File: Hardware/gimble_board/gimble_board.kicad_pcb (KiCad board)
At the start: 2 copper layers, 124.5 x 95.9 mm, 97 parts, among them J1 Test_Point, J2 Test_Point, J3 Test_Point, J4 Test_Point, Q1 Q_NMOS_GDS, Q2 Q_NMOS_GDS, Q3 Q_NMOS_GDS, Q4 Q_NMOS_GDS, Q5 Q_NMOS_GDS, Q6 Q_NMOS_GDS, Q7 Q_NMOS_GDS, Q8 Q_NMOS_GDS, SW1 SW_Push, SW2 SW_Push, SW3 SW_Push, SW4 SW_Push, SW5 SW_Push, SW6 SW_Push, SW7 SW_Push, SW8 SW_Push, SW9 SW_SPDT, U1 LM2576SX-3.3, U2 LM2576SX-5.0, U3 TM4C129E_Launchpad

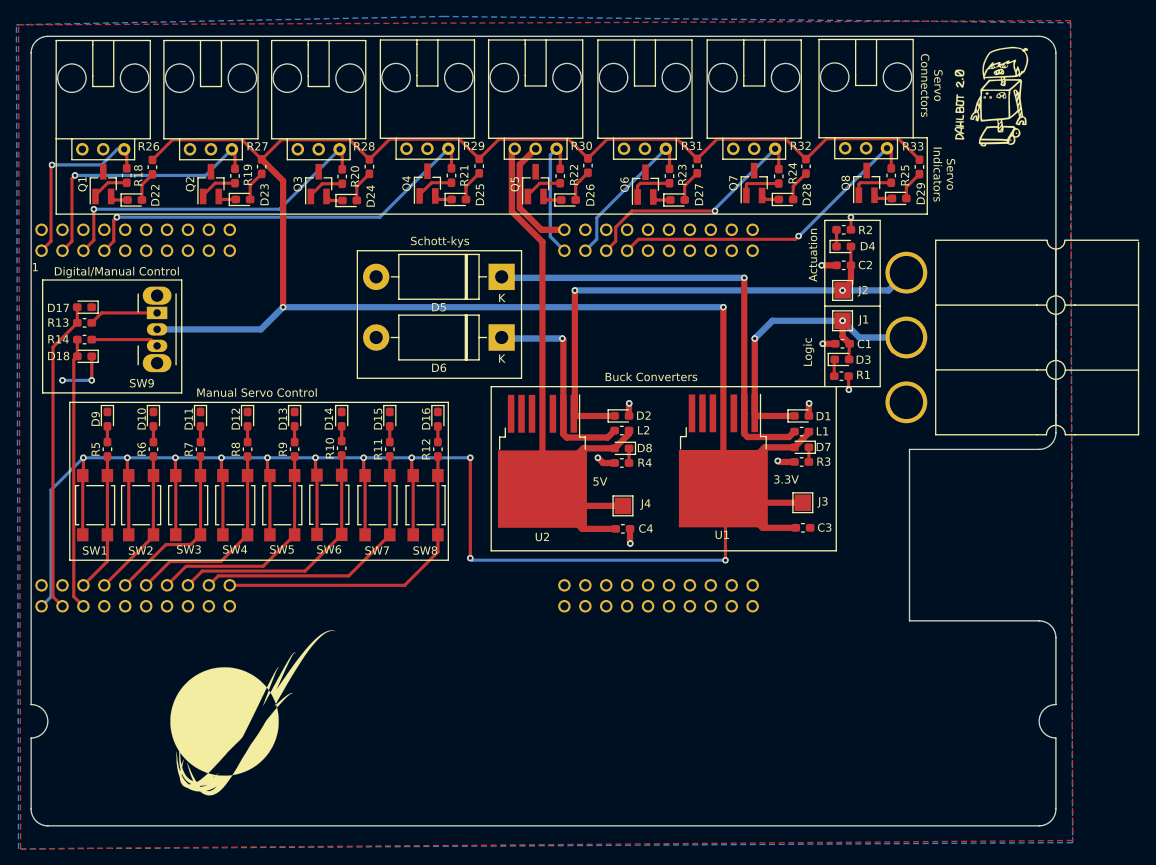
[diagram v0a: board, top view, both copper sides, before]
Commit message: layout 9
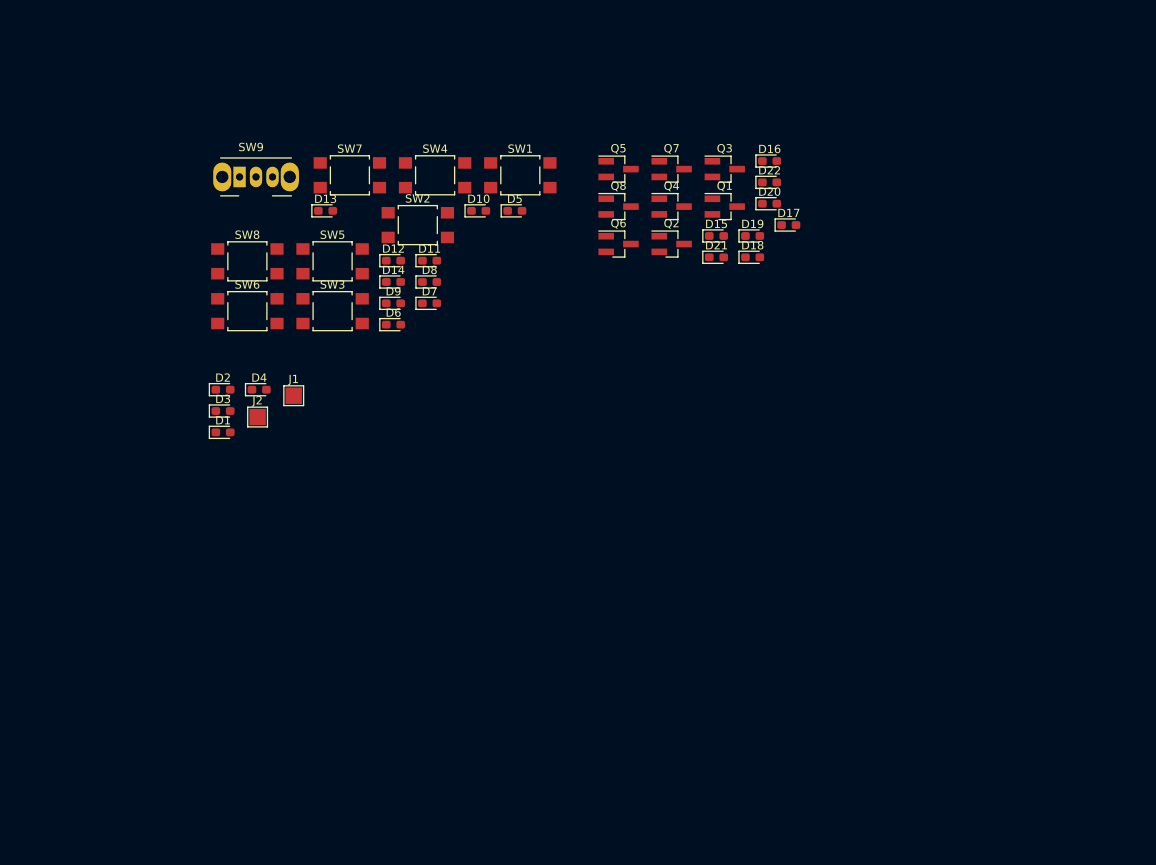
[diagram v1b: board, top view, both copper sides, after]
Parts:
- removed C1, C2: 100uF, Capacitor_SMD:C_0603_1608Metric_Pad1.05x0.95mm_HandSolder
- removed C3, C4: 1000uF, Capacitor_SMD:C_0603_1608Metric_Pad1.05x0.95mm_HandSolder
- removed Conn1: AndersonPP, MRDT_Connectors:Anderson_3_Horizontal_Side_by_Side
- removed Conn2, Conn3, Conn4, Conn5, Conn6, Conn7, Conn8, Conn9: Molex_SL_03, MRDT_Connectors:MOLEX_SL_03_Horizontal
- removed D23, D24, D25, D26, D27, D28, D29: LED, LED_SMD:LED_0603_1608Metric_Pad1.05x0.95mm_HandSolder
- removed G***: LOGO, MRDT_Silkscreens:0_MRDT_Logo_20mm
- removed G***: LOGO, MRDT_Silkscreens:2_Dahlbot_2.0
- removed J3, J4: Test_Point, TestPoint:TestPoint_Pad_2.0x2.0mm
- removed L1, L2: 100uH, Inductor_SMD:L_0603_1608Metric_Pad1.05x0.95mm_HandSolder
- removed R1, R2: 1k, Resistor_SMD:R_0603_1608Metric_Pad1.05x0.95mm_HandSolder
- removed R10, R11, R12, R13, R14, R26, R27, R28, R29, R3, R30, R31, R32, R33, R5, R6, R7, R8, R9: 330, Resistor_SMD:R_0603_1608Metric_Pad1.05x0.95mm_HandSolder
- removed R18, R19, R20, R21, R22, R23, R24, R25, R4: 500, Resistor_SMD:R_0603_1608Metric_Pad1.05x0.95mm_HandSolder
- removed U1: LM2576SX-3.3, Package_TO_SOT_SMD:TO-263-6
- removed U2: LM2576SX-5.0, Package_TO_SOT_SMD:TO-263-6
- removed U3: TM4C129E_Launchpad, MRDT_Shields:TM4C129E_Launchpad_FULL_THT_BOTTOM
- added D19: LED, LED_SMD:LED_0603_1608Metric_Pad1.05x0.95mm_HandSolder, F.Cu at (151.1, 52.8)
- added D20: LED, LED_SMD:LED_0603_1608Metric_Pad1.05x0.95mm_HandSolder, F.Cu at (153.2, 48.9)
- added D21: LED, LED_SMD:LED_0603_1608Metric_Pad1.05x0.95mm_HandSolder, F.Cu at (146.7, 55.4)
- D5, D6: value D_Schottky -> LED; footprint Diode_THT:D_DO-201AD_P15.24mm_Horizontal -> LED_SMD:LED_0603_1608Metric_Pad1.05x0.95mm_HandSolder
- moved D17 86.1 mm to (155.5, 51.5), turned to 0 degrees
- moved D18 82.0 mm to (151.1, 55.4), turned to 0 degrees
- moved D22 77.1 mm to (153.2, 46.3)
- moved Q1 75.5 mm to (147.7, 49.3), turned to 0 degrees
- moved D3 75.4 mm to (86.8, 74.1)
- moved D4 73.1 mm to (91.2, 71.5)
- moved J2 72.7 mm to (91.0, 74.8)
- moved D1 70.3 mm to (86.8, 76.7)
- moved J1 67.3 mm to (95.4, 72.2)
- moved SW1 65.4 mm to (122.9, 45.5), turned to 0 degrees
- moved Q2 56.4 mm to (141.3, 53.8), turned to 0 degrees
- moved D16 51.0 mm to (153.2, 43.7), turned to 0 degrees
- moved Q3 49.4 mm to (147.7, 44.7), turned to 0 degrees
- moved D2 48.5 mm to (86.8, 71.5)
- moved D7 48.5 mm to (111.9, 61.0), turned to 0 degrees
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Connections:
- D13 pad 2: Net-(D13-Pad2) -> Servo_Digital_Control
- D14 pad 2: Net-(D14-Pad2) -> Servo_Manual_Control
- D15 pad 1: GND -> Net-(D15-Pad1)
- D16 pad 1: GND -> Net-(D16-Pad1)
- D17 pad 1: GND -> Net-(D17-Pad1)
- D17 pad 2: Servo_Digital_Control -> Net-(D17-Pad2)
- D18 pad 1: GND -> Net-(D18-Pad1)
- D18 pad 2: Servo_Manual_Control -> Net-(D18-Pad2)
- D5 pad 1: Net-(D5-Pad1) -> GND
- D5 pad 2: GND -> Net-(D5-Pad2)
- D6 pad 1: Net-(D6-Pad1) -> GND
- D6 pad 2: GND -> Net-(D6-Pad2)
- D7 pad 1: Net-(D7-Pad1) -> GND
- D7 pad 2: +3V3 -> Net-(D7-Pad2)
- D8 pad 1: Net-(D8-Pad1) -> GND
- D8 pad 2: +5V -> Net-(D8-Pad2)
- Q1 pad 2: Net-(D22-Pad1) -> Net-(D15-Pad1)
- Q2 pad 2: Net-(D23-Pad1) -> Net-(D16-Pad1)
- Q3 pad 2: Net-(D24-Pad1) -> Net-(D17-Pad1)
- Q4 pad 2: Net-(D25-Pad1) -> Net-(D18-Pad1)
- Q8 pad 2: Net-(D29-Pad1) -> Net-(D22-Pad1)
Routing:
- net +3V3: track 449.7 -> 0.00 mm, vias 13 -> 0
- net +5V: track 86.1 -> 0.00 mm
- net Power_Input_Act: track 67.0 -> 0.00 mm, vias 2 -> 0
- net Net-(D5-Pad1): track 55.0 -> 0.00 mm, vias 1 -> 0
- net Servo_4_PWM: track 50.9 -> 0.00 mm, vias 1 -> 0
- net Power_Input_Log: track 43.5 -> 0.00 mm, vias 2 -> 0
- net Servo_3_PWM: track 41.0 -> 0.00 mm, vias 1 -> 0
- net Servo_8_AW: track 39.4 -> 0.00 mm, vias 1 -> 0
- net Servo_8_SW: track 38.6 -> 0.00 mm
- net Servo_Digital_Control: track 38.0 -> 0.00 mm
- net GND: track 37.1 -> 0.00 mm, vias 11 -> 0
- net Servo_7_SW: track 34.0 -> 0.00 mm
- net Servo_Manual_Control: track 33.0 -> 0.00 mm
- net Servo_2_PWM: track 32.7 -> 0.00 mm, vias 1 -> 0
- net Servo_6_SW: track 30.8 -> 0.00 mm
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- removed copper zone on B.Cu, net +5V
- removed copper zone on F.Cu, net GND
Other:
- board outline removed
- board text removed: "3.3V"
- board text removed: "5V"
- board text removed: "Actuation"
- board text removed: "Buck Converters"
- board text removed: "Digital/Manual Control"
- board text removed: "Logic"
- board text removed: "Manual Servo Control"
- board text removed: "Schott-kys"
- board text removed: "Servo Connectors"
- board text removed: "Servo Indicators"
